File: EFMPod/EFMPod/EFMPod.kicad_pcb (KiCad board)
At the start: 2 copper layers, 61 x 35.6 mm, 51 parts, among them J1 Conn_02x05_Odd_Even, J2 UJ2-MBH-1-SMT-TR, J3 Conn_02x18_Odd_Even, SW1 SW_Push, SW2 SW_Push, SW3 SW_Push, U1 AZ1117CH-3_3TRG1, U2 EFM32HG322F64, Y1 24MHz, Y2 Crystal_GND3

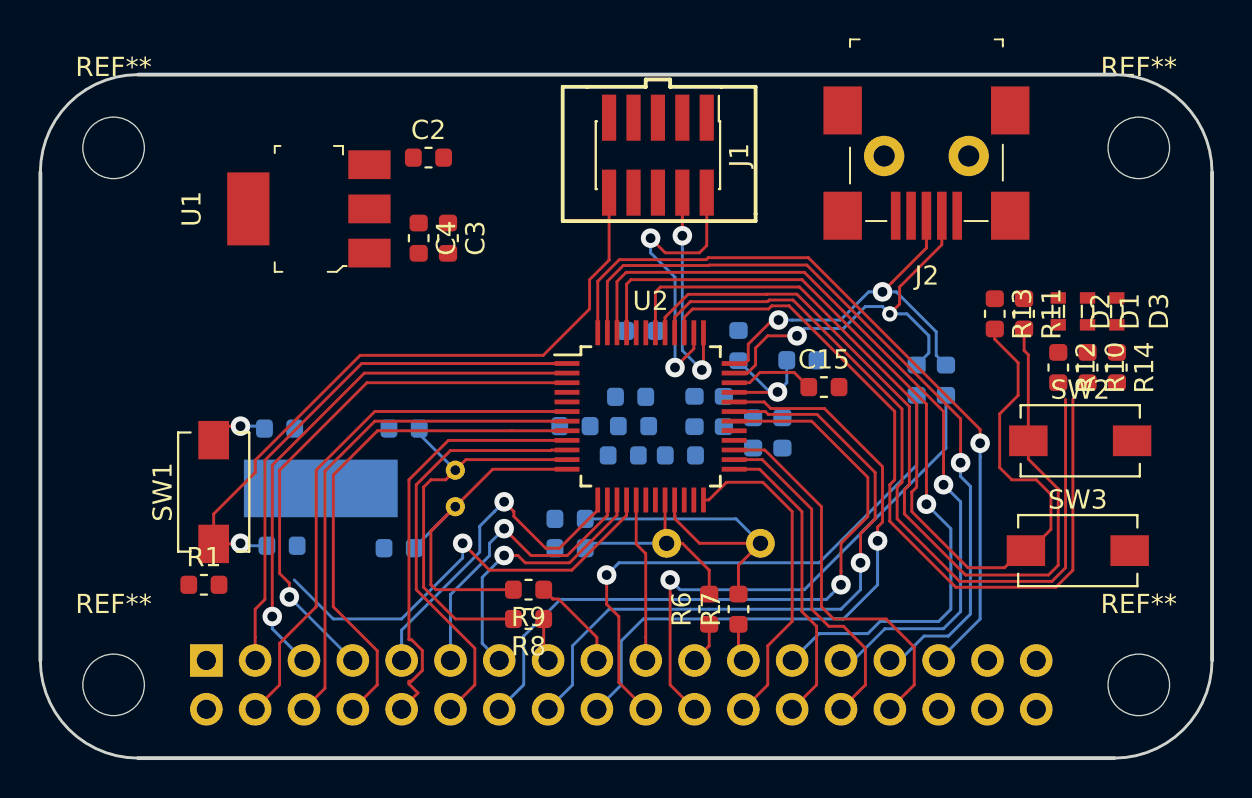
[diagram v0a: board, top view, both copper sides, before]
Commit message: Layout done
Layout done, silk & gerbers next
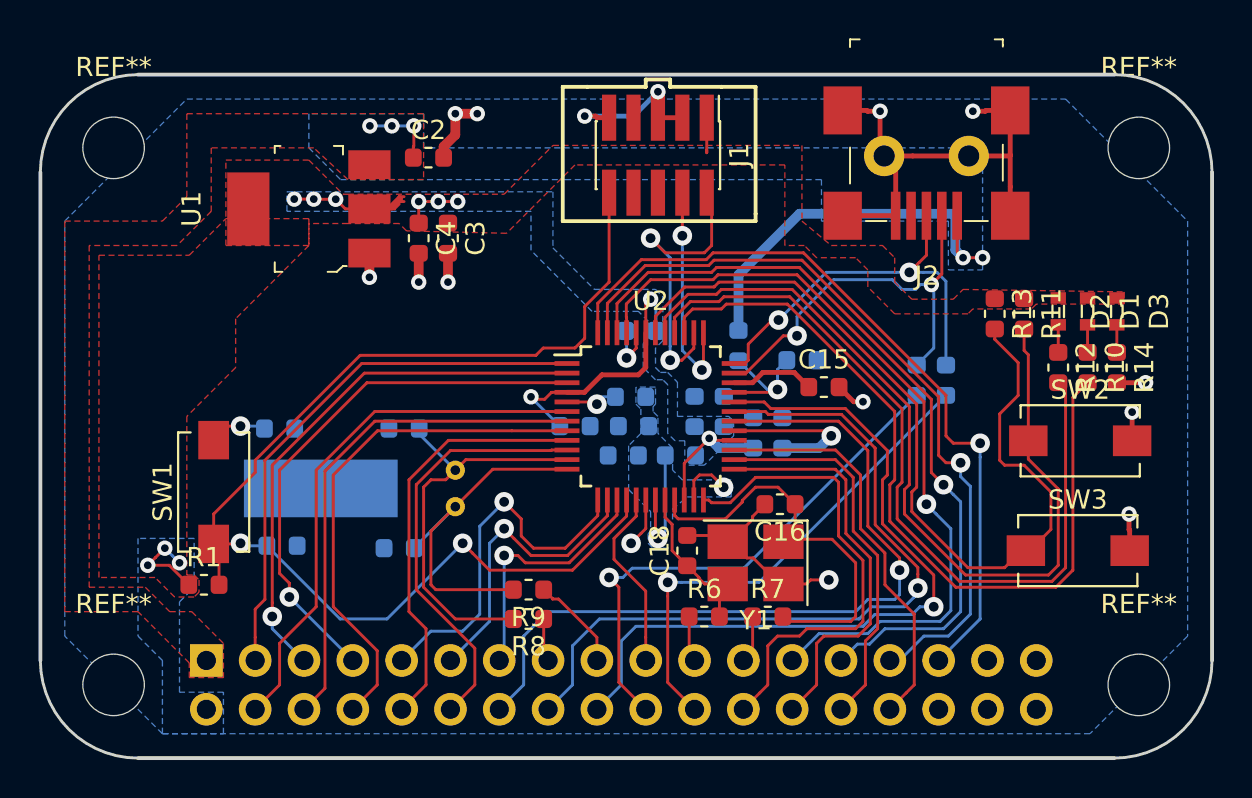
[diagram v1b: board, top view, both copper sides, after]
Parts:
- C16, C18: moved to F.Cu
- Y1: value 24MHz -> Crystal_GND24; footprint Crystal:Crystal_HC49-U_Vertical -> Crystal:Crystal_SMD_SeikoEpson_FA238-4Pin_3.2x2.5mm_HandSoldering; moved to F.Cu
- moved C16 10.9 mm to (164.2, 89.7)
- moved C18 6.10 mm to (159.4, 92.1), turned to 90 degrees
- moved R7 1.57 mm to (163.6, 95.5), turned to 0 degrees
- moved Y1 1.05 mm to (162.9, 92.7)
- moved R6 0.46 mm to (160.3, 95.5), turned to 0 degrees
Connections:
- Y1 pad 2: /XTALP -> GNDREF
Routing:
- net GNDREF: track 0.00 -> 66.9 mm, vias 0 -> 17
- net +3V3: track 0.00 -> 42.9 mm, vias 0 -> 12
- net VBUS: track 0.00 -> 25.2 mm, vias 0 -> 5
- net Net-(C12-Pad1): track 0.00 -> 9.49 mm, vias 0 -> 2
- net Net-(C14-Pad1): track 0.00 -> 7.96 mm, vias 0 -> 1
- net /PD4: track 17.0 -> 24.8 mm
- net /PD5: track 15.6 -> 21.2 mm
- net /PC10: track 34.0 -> 39.4 mm
- net /~EFM_RESET: track 58.0 -> 62.7 mm
- net /PC9: track 35.1 -> 39.5 mm
- net /PC8: track 36.3 -> 40.6 mm
- net /XTALM: track 18.7 -> 21.7 mm
- net /PC14: track 30.0 -> 27.6 mm
- net /PD6: track 17.6 -> 20.0 mm
- net /XTALP: track 10.7 -> 8.42 mm
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- added copper zone on B.Cu, net +3V3
- added copper zone on F.Cu, net +3V3
- added copper zone on B.Cu, net GNDREF
- added copper zone on B.Cu, net Net-(C12-Pad1)
- added copper zone on B.Cu, net VBUS
- added copper zone on F.Cu, net VBUS
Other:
- net class Power: clearance 0.254 -> 2.032; trace_width 0.254 -> 2.032
